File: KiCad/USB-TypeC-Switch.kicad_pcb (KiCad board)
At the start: 4 copper layers, 48.5 x 50 mm, 59 parts, among them J1 USB_C_IN_1, J2 USB_C_IN_2, J3 USB_C_OUT, J4 Conn_02x05_Odd_Even, SW1 SW_Push, U1 FUSB340TMX, U2 FUSB340TMX, U3 NL3S588, U4 AP63205WU, U5 UCS3205-E_Q8A, U6 UCS3205-E_Q8A, U7 NL3S588, U8 AZ1117C-3.3, U9 ATSAMD21E15B-M

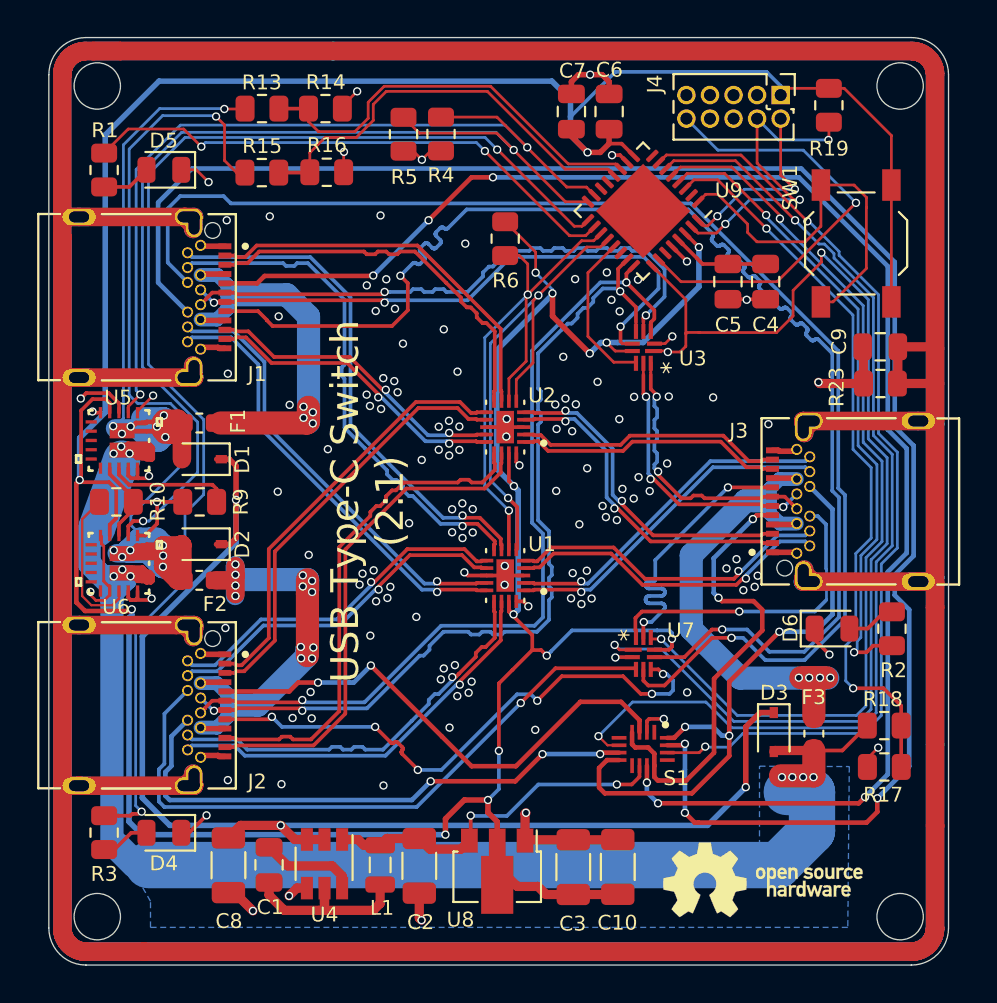
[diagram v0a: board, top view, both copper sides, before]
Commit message: Migrate to KiCad 6.x
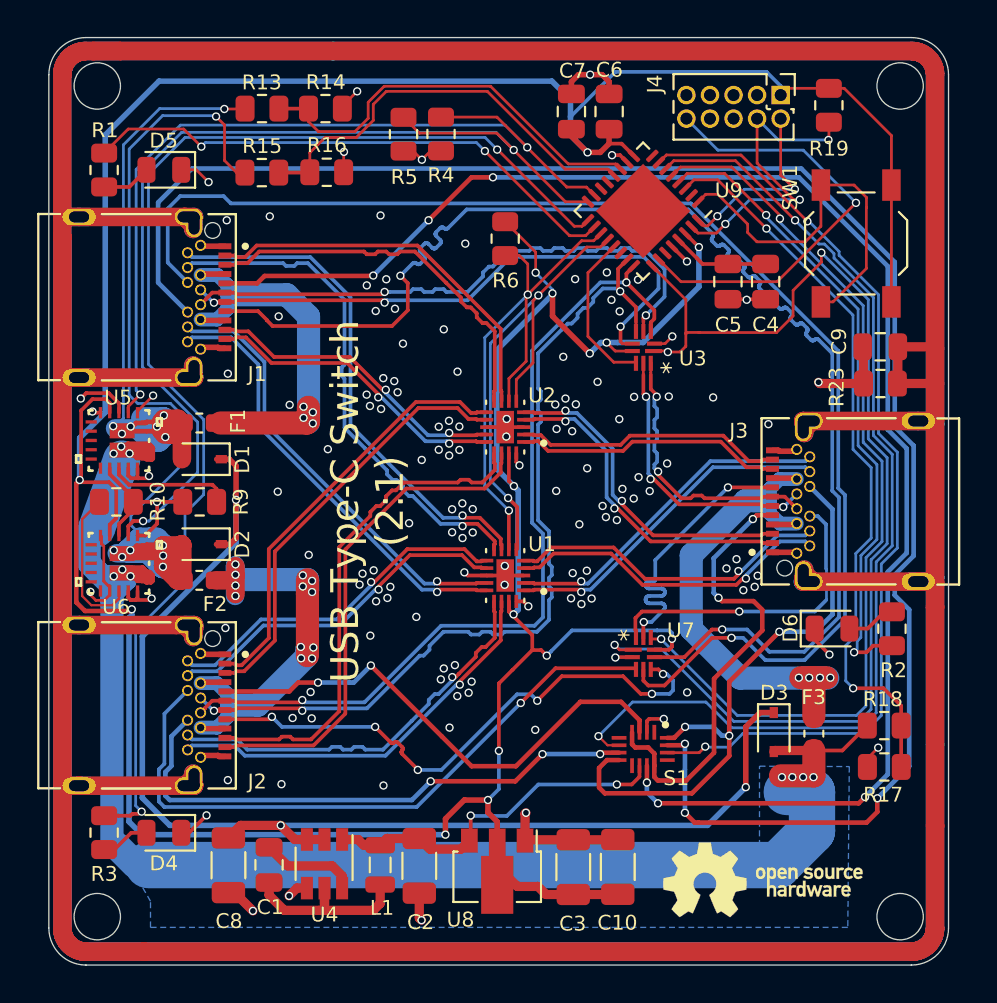
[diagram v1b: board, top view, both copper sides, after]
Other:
- net class Default removed
- net class GNDS removed
- net class USB2_90ohm removed
- net class USB3_90ohm removed
- net class VBUS removed
- net class low_speed_diff removed
